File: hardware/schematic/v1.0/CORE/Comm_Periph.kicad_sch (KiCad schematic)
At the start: 20 parts, among them J1 Conn_01x06_Socket, J10 USB_C_Receptacle_USB2.0_16P, J11 Conn_01x06_Socket, J14 Conn_01x03_Socket, J15 Conn_01x05_Socket, U6 CH340E

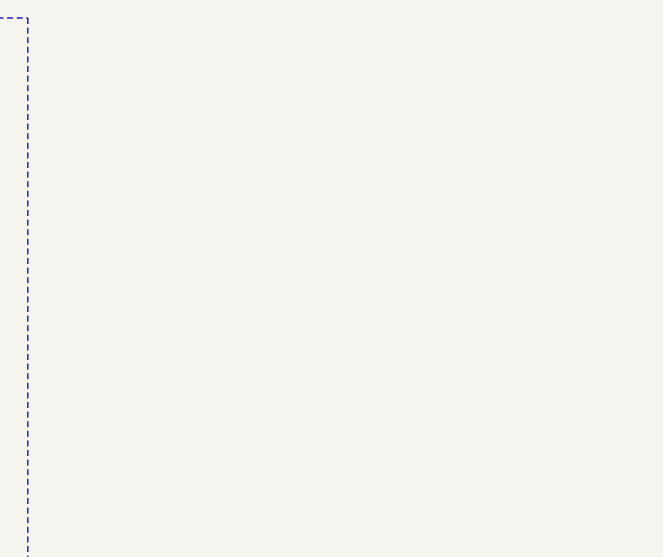
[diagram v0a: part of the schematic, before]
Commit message: sch update
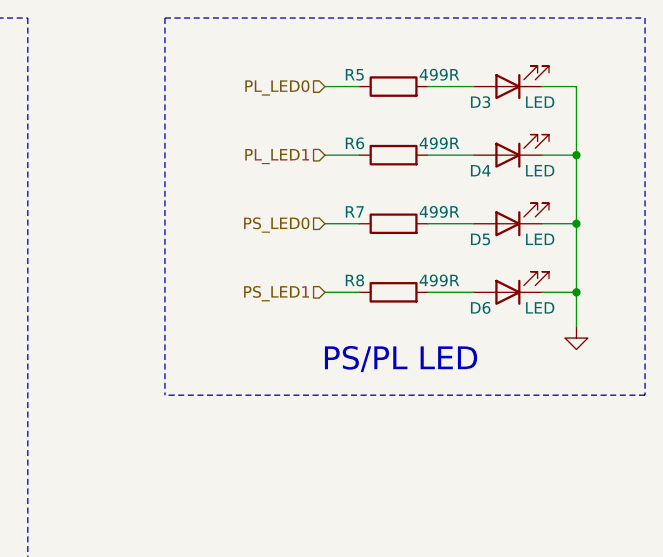
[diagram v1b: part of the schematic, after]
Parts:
- added D3, D4, D5, D6: LED, LED_SMD:LED_0603_1608Metric, symbol Device:LED
- added R5, R6, R7, R8: 499R, Resistor_SMD:R_0402_1005Metric, symbol Device:R
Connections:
- net GND: now also D3.1 (K), D4.1 (K), D5.1 (K), D6.1 (K)
- new net: D4.2 (A), R6.2
- new net: D6.2 (A), R8.2
- new net: D5.2 (A), R7.2
- new net: D3.2 (A), R5.2
- new net PL_LED0: R5.1
- new net PL_LED1: R6.1
- new net PS_LED0: R7.1
- new net PS_LED1: R8.1
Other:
- note added: "PS/PL LED"

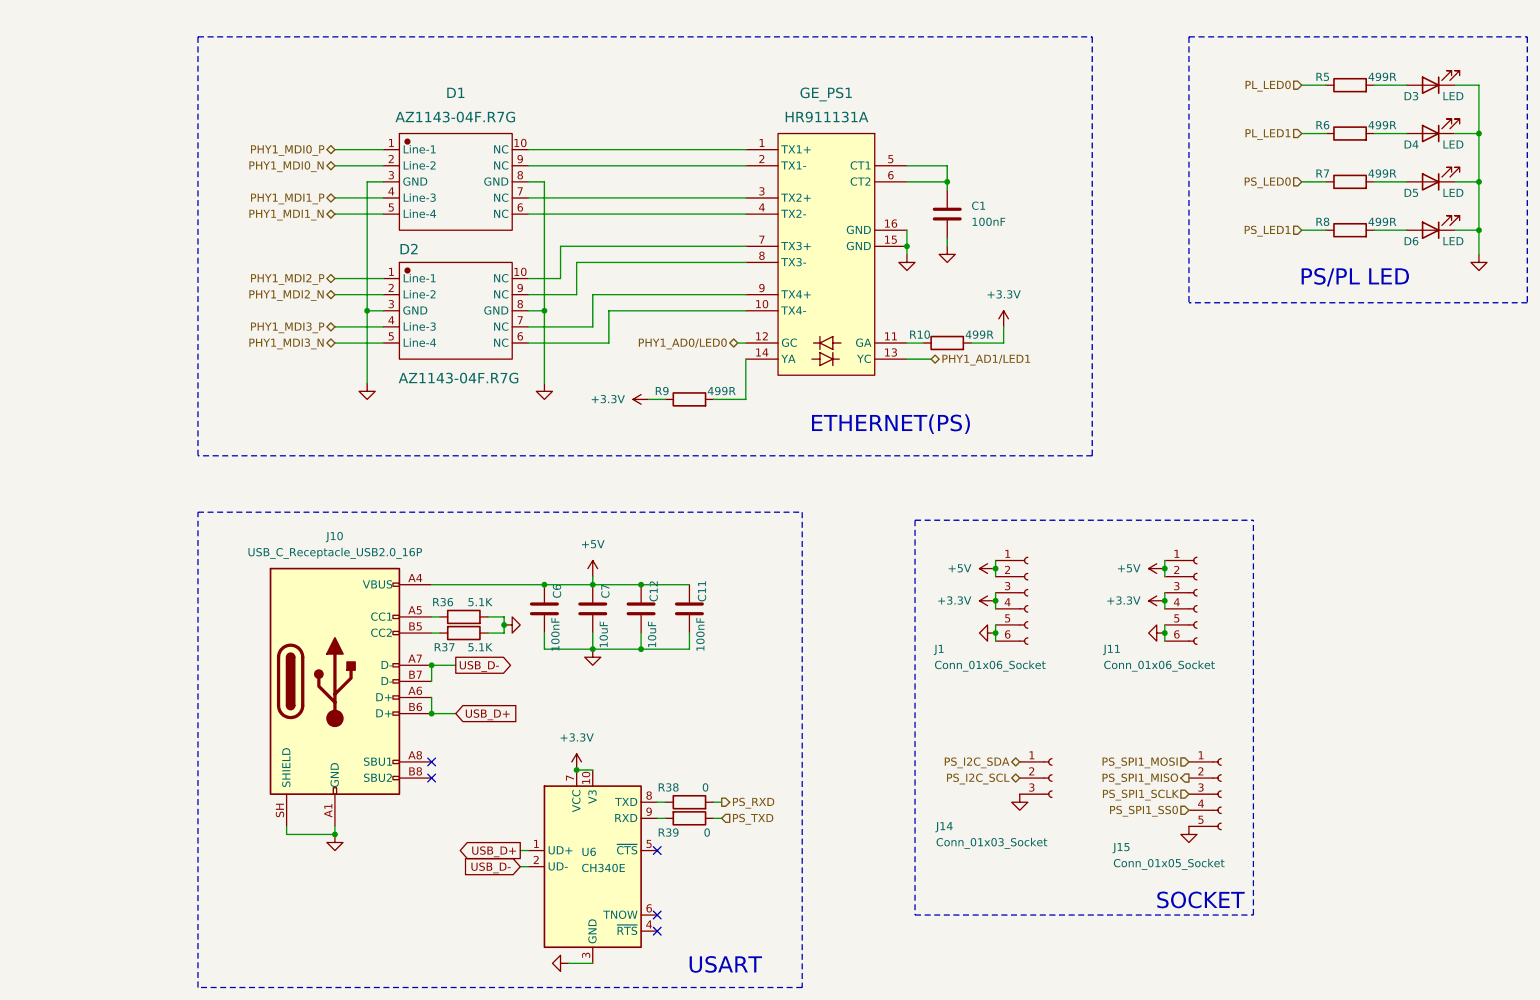
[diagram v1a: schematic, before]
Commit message: sch update
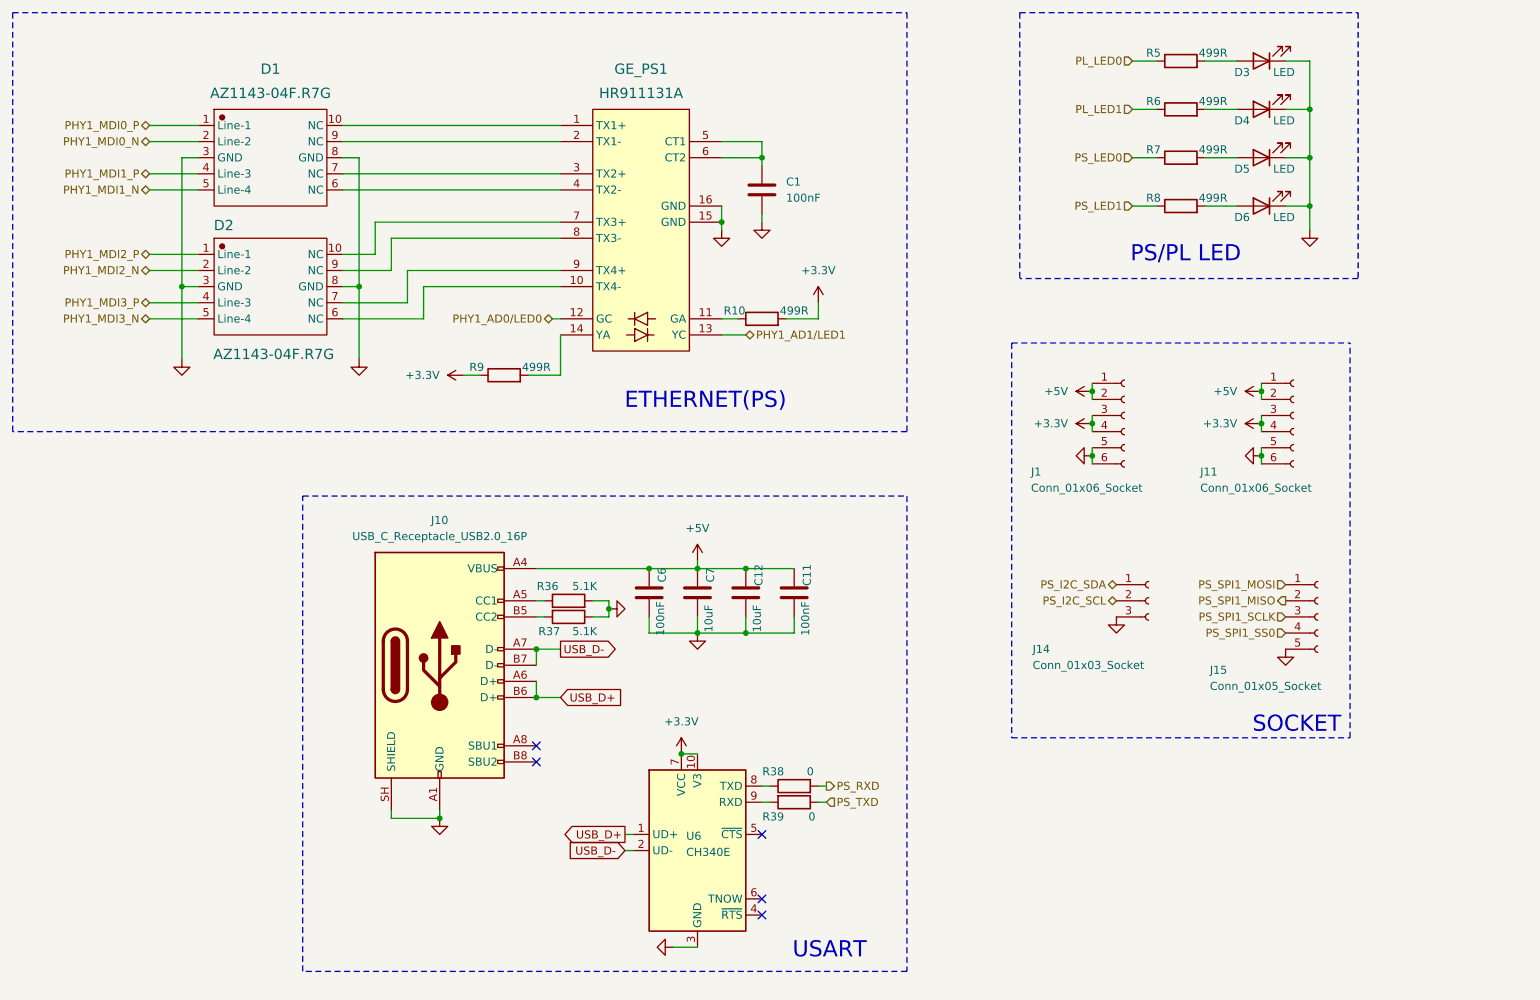
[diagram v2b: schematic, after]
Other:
- moved on the sheet: C1, C11, C12, C6, C7, D1, D2, D3, D4, D5, D6, GE_PS1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

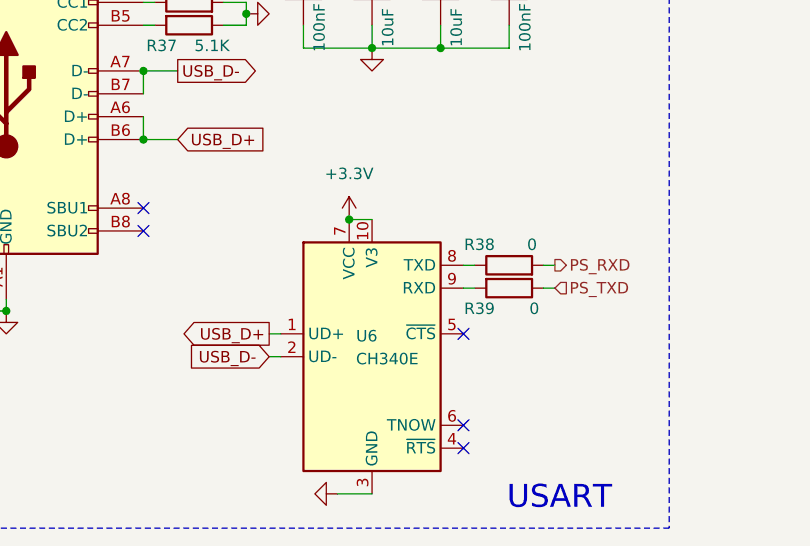
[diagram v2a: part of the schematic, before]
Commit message: sch update
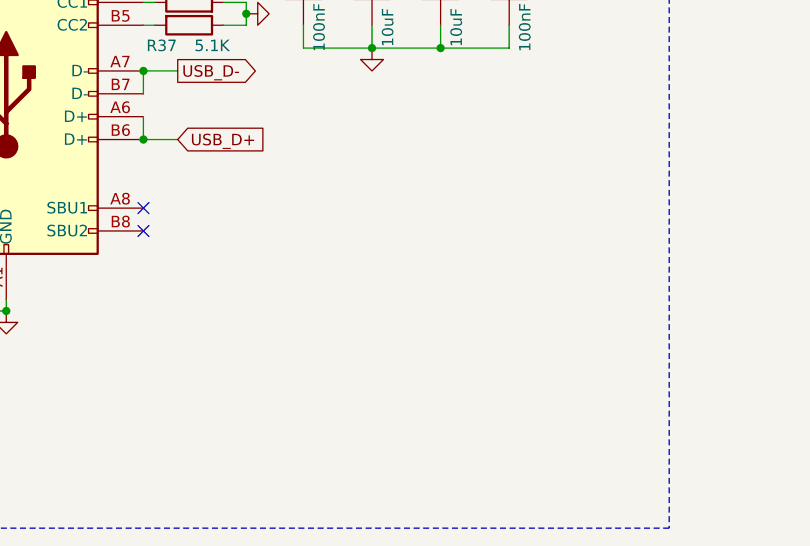
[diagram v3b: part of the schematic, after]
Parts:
- removed R38, R39: 0, Resistor_SMD:R_0402_1005Metric, symbol Device:R
- removed U6: CH340E, Package_SO:MSOP-10_3x3mm_P0.5mm, symbol Interface_USB:CH340E
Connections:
- no-connect marks 5 -> 2
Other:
- note removed: "USART"

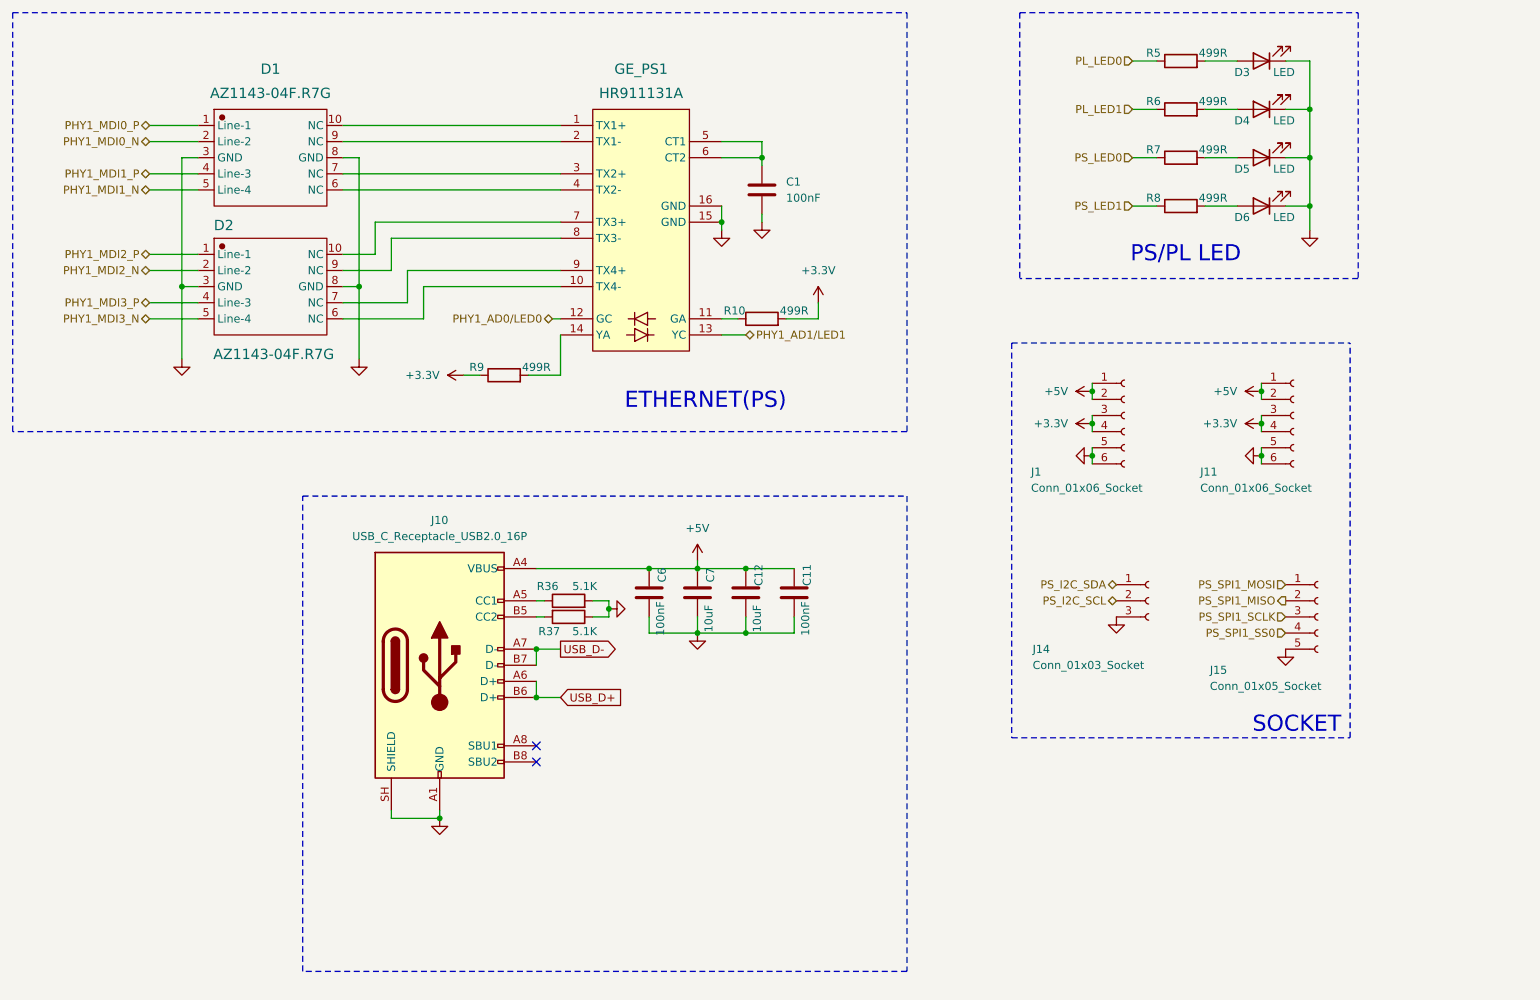
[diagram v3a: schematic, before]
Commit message: sch update
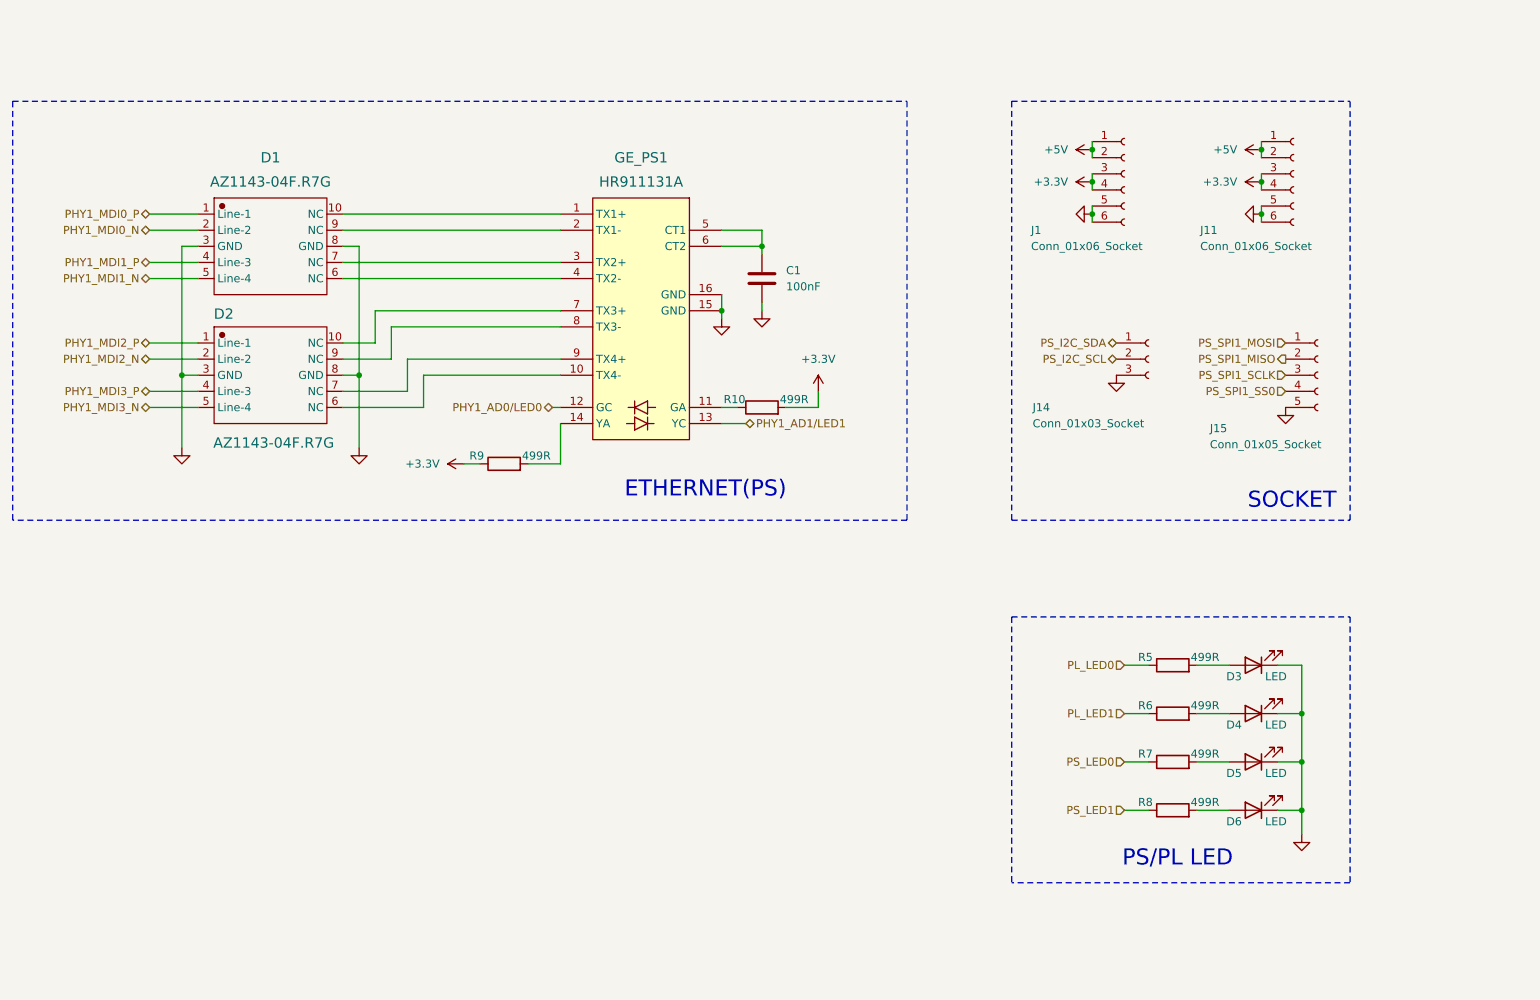
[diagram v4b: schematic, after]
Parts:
- removed C11, C6: 100nF, Capacitor_SMD:C_0402_1005Metric, symbol Device:C
- removed C12, C7: 10uF, Capacitor_SMD:C_0603_1608Metric, symbol Device:C
- removed J10: USB_C_Receptacle_USB2.0_16P, Connector_USB:USB_C_Receptacle_Palconn_UTC16-G, symbol Connector:USB_C_Receptacle_USB2.0_16P
- removed R36, R37: 5.1K, Resistor_SMD:R_0402_1005Metric, symbol Device:R
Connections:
- no-connect marks 2 -> 0
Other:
- moved on the sheet: C1, D1, D2, D3, D4, D5, D6, GE_PS1, J1, J11, J14, J15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

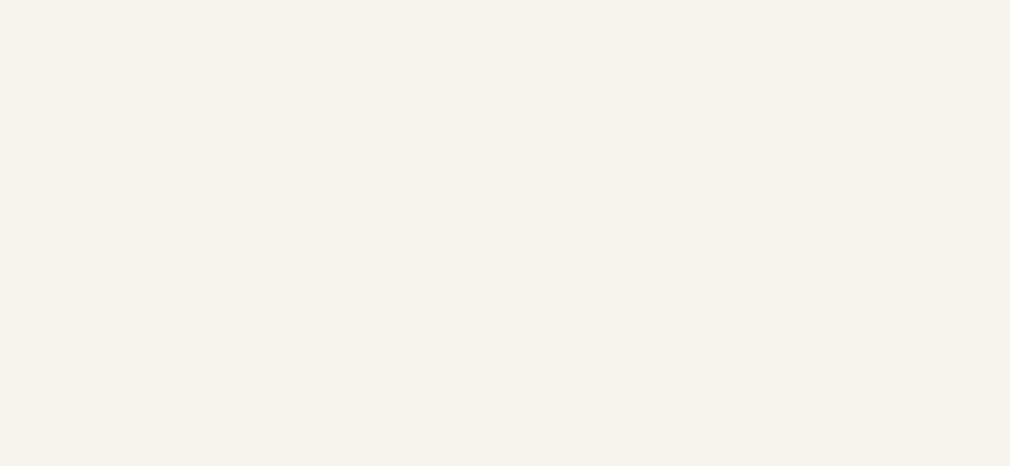
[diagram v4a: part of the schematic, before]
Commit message: sch update
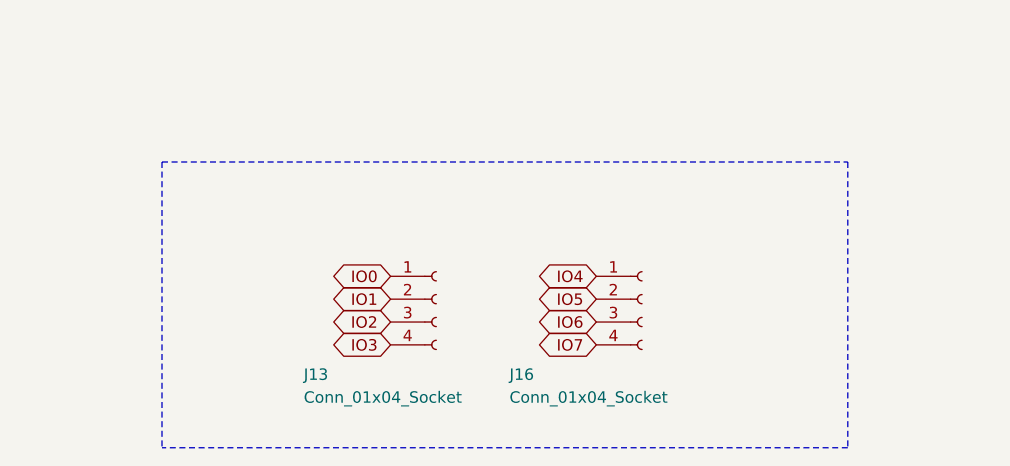
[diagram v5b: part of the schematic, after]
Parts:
- added J13, J16: Conn_01x04_Socket, Connector_PinHeader_2.54mm:PinHeader_1x04_P2.54mm_Vertical, symbol Connector:Conn_01x04_Socket
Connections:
- new net IO0: J13.1 (Pin_1)
- new net IO1: J13.2 (Pin_2)
- new net IO2: J13.3 (Pin_3)
- new net IO3: J13.4 (Pin_4)
- new net IO4: J16.1 (Pin_1)
- new net IO5: J16.2 (Pin_2)
- new net IO6: J16.3 (Pin_3)
- new net IO7: J16.4 (Pin_4)
